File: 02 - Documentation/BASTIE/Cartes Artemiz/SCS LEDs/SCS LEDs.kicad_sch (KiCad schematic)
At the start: 18 parts, among them J1 2P Droit 2-11-2022, J2 2P Droit 2-11-2022, K1 SSR CPC1394GR, U1 ${SIM.PARAMS}, U2 Opamp_Dual, U3 Alim LP TSR_0.5-2450

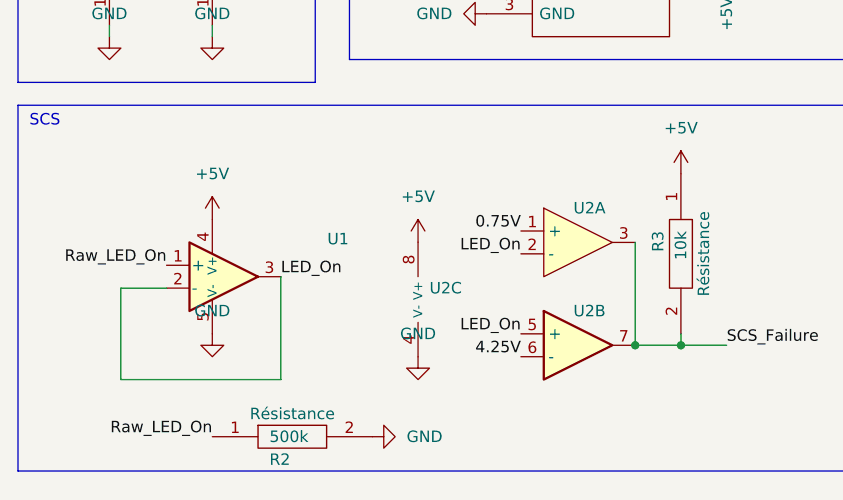
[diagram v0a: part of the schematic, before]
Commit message: Kicadlib + Modifs cartes
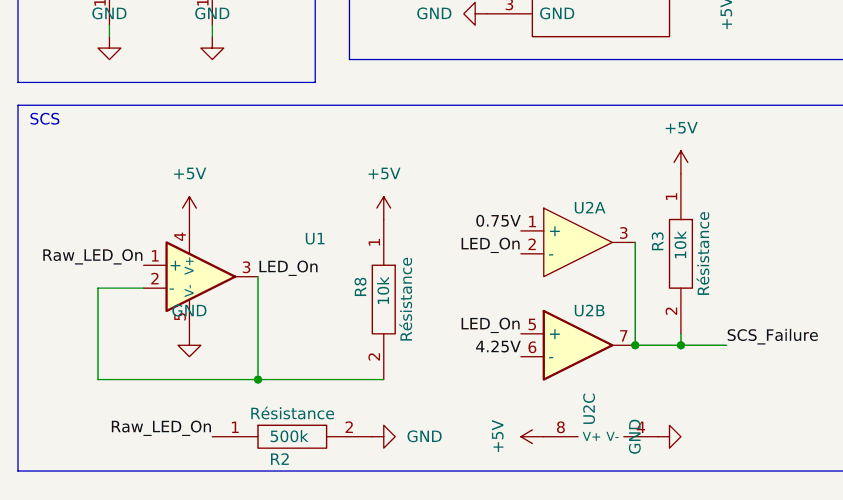
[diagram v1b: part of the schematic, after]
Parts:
- added R8: 10k, EPSA_lib:RESC3216X70N, symbol EPSA_lib:Résistance RK73H2BLTDD2152F
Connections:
- net +5V: now also R8.1
- net LED_On: now also R8.2
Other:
- moved on the sheet: U1, U2C
